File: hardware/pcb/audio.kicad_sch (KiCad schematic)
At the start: 27 parts, among them J400 AudioJack3_SwitchT, U400 CS43130, U401 ADP150-1.8, U402 ADP150-1.8, Y400 22.5792MHz

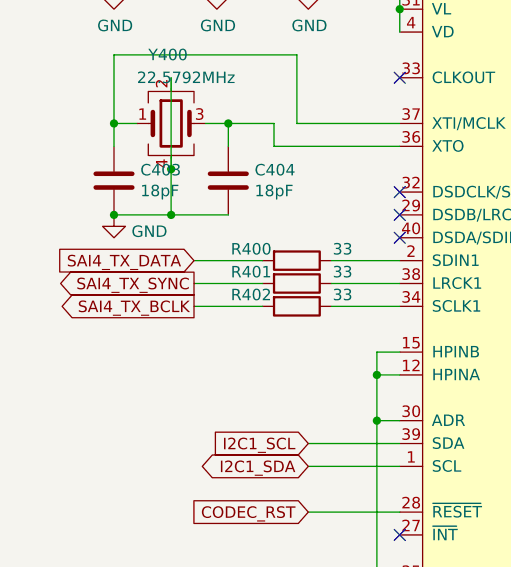
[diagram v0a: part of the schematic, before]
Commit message: - Working on pcb layout
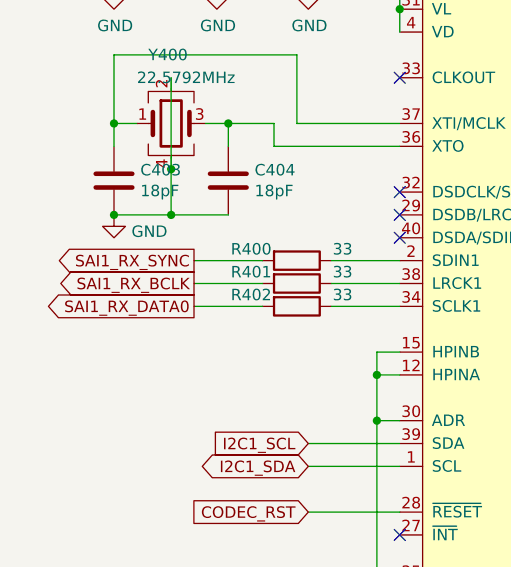
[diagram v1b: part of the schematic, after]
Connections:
- net SAI4_TX_BCLK renamed SAI1_RX_DATA0
- net SAI4_TX_DATA renamed SAI1_RX_SYNC
- net SAI4_TX_SYNC renamed SAI1_RX_BCLK
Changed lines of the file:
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@@
     (stroke (width 0) (type solid) (color 0 0 0 0))
   )
-  (global_label "SAI4_TX_DATA" (shape input) (at 177.8 149.86 180)
+  (global_label "SAI1_RX_SYNC" (shape output) (at 177.8 149.86 180)
     (effects (font (size 1.27 1.27)) (justify right))
-    (property "Intersheet References" "${INTERSHEET_REFS}" (id 0) (at 161.2234 149.7806 0)
+    (property "Intersheet References" "${INTERSHEET_REFS}" (id 0) (at 160.4372 149.7806 0)
       (effects (font (size 1.27 1.27)) (justify right) hide)
     )
   )
-  (global_label "SAI4_TX_SYNC" (shape output) (at 177.8 152.4 180)
+  (global_label "SAI1_RX_BCLK" (shape output) (at 177.8 152.4 180)
     (effects (font (size 1.27 1.27)) (justify right))
-    (property "Intersheet References" "${INTERSHEET_REFS}" (id 0) (at 160.7396 152.3206 0)
+    (property "Intersheet References" "${INTERSHEET_REFS}" (id 0) (at 160.4977 152.3206 0)
       (effects (font (size 1.27 1.27)) (justify right) hide)
     )
   )
-  (global_label "SAI4_TX_BCLK" (shape output) (at 177.8 154.94 180)
+  (global_label "SAI1_RX_DATA0" (shape output) (at 177.8 154.94 180)
     (effects (font (size 1.27 1.27)) (justify right))
-    (property "Intersheet References" "${INTERSHEET_REFS}" (id 0) (at 160.8 154.8606 0)
+    (property "Intersheet References" "${INTERSHEET_REFS}" (id 0) (at 159.7115 154.8606 0)
       (effects (font (size 1.27 1.27)) (justify right) hide)
     )

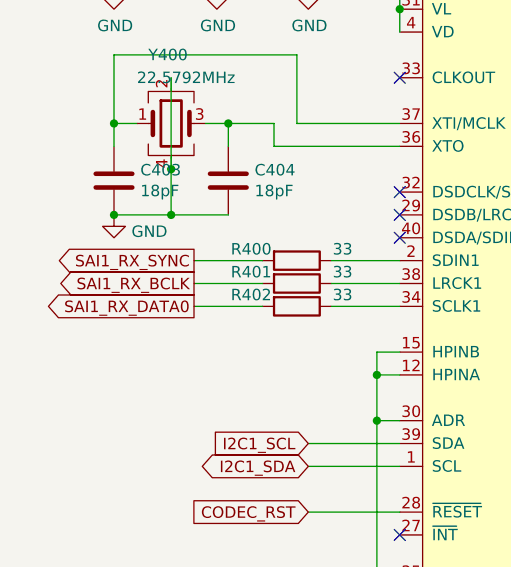
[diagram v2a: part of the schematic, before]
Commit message: - PCB: prepare for r0p4
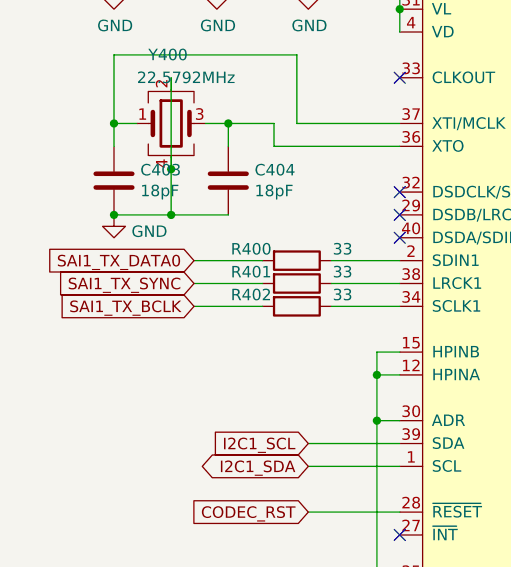
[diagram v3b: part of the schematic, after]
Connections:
- net SAI1_RX_BCLK renamed SAI1_TX_SYNC
- net SAI1_RX_DATA0 renamed SAI1_TX_BCLK
- net SAI1_RX_SYNC renamed SAI1_TX_DATA0
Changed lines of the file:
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@@
     (stroke (width 0) (type solid) (color 0 0 0 0))
   )
-  (global_label "SAI1_RX_SYNC" (shape output) (at 177.8 149.86 180)
+  (global_label "SAI1_TX_DATA0" (shape input) (at 177.8 149.86 180)
     (effects (font (size 1.27 1.27)) (justify right))
-    (property "Intersheet References" "${INTERSHEET_REFS}" (id 0) (at 160.4372 149.7806 0)
+    (property "Intersheet References" "${INTERSHEET_REFS}" (id 0) (at 160.0139 149.7806 0)
       (effects (font (size 1.27 1.27)) (justify right) hide)
     )
   )
-  (global_label "SAI1_RX_BCLK" (shape output) (at 177.8 152.4 180)
+  (global_label "SAI1_TX_SYNC" (shape input) (at 177.8 152.4 180)
     (effects (font (size 1.27 1.27)) (justify right))
-    (property "Intersheet References" "${INTERSHEET_REFS}" (id 0) (at 160.4977 152.3206 0)
+    (property "Intersheet References" "${INTERSHEET_REFS}" (id 0) (at 160.7396 152.3206 0)
       (effects (font (size 1.27 1.27)) (justify right) hide)
     )
   )
-  (global_label "SAI1_RX_DATA0" (shape output) (at 177.8 154.94 180)
+  (global_label "SAI1_TX_BCLK" (shape input) (at 177.8 154.94 180)
     (effects (font (size 1.27 1.27)) (justify right))
-    (property "Intersheet References" "${INTERSHEET_REFS}" (id 0) (at 159.7115 154.8606 0)
+    (property "Intersheet References" "${INTERSHEET_REFS}" (id 0) (at 160.8 154.8606 0)
       (effects (font (size 1.27 1.27)) (justify right) hide)
     )
